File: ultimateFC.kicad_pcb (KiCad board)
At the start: 6 copper layers, 36 x 36 mm, 240 parts, among them J1 USB_B_Micro, SW1 SW_Push, U1 LMR33630CQRNX, U2 TPS62824ADMQ, U3 LMR33620CRNXT, U4 S25FL064L, U5 DPS310, U6 BMI270, U7 STM32H735VGH6, U8 ICM-20602, Y1 CSTNE8M00G550000R0

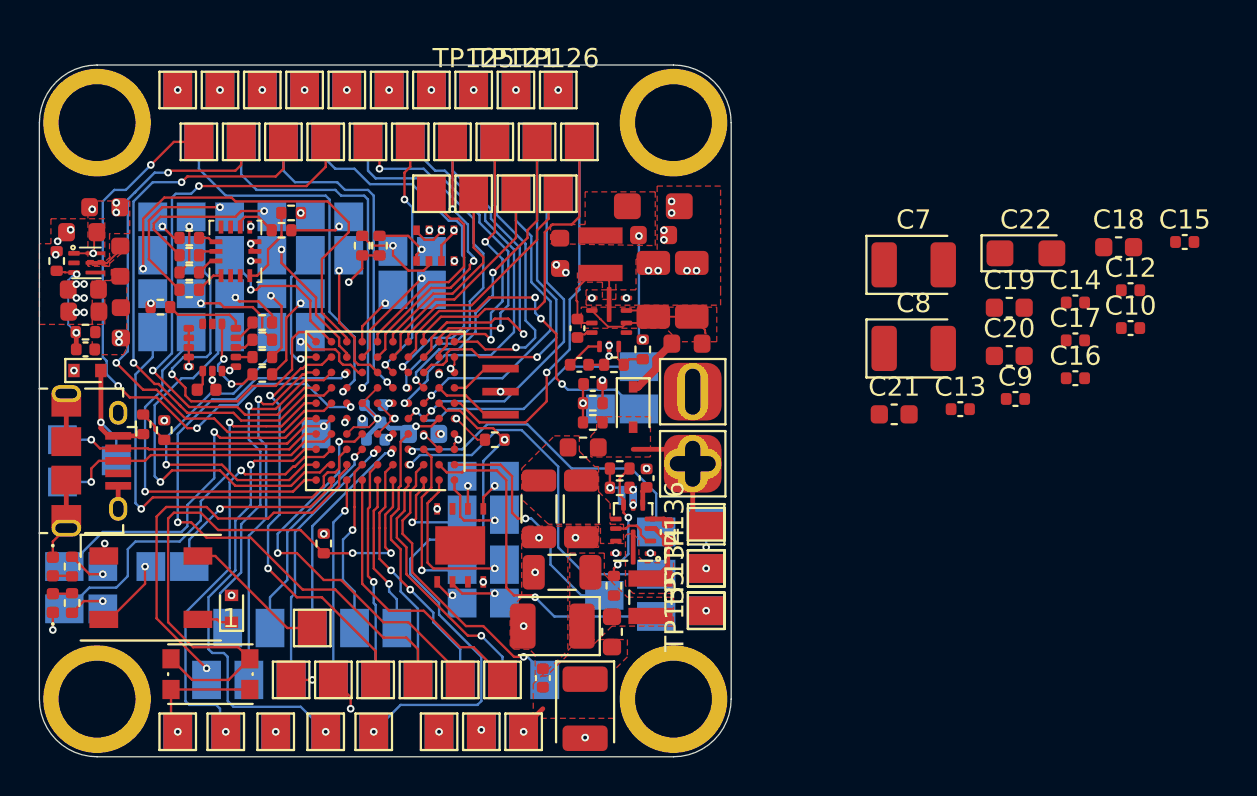
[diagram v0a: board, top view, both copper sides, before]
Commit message: layout tweaks
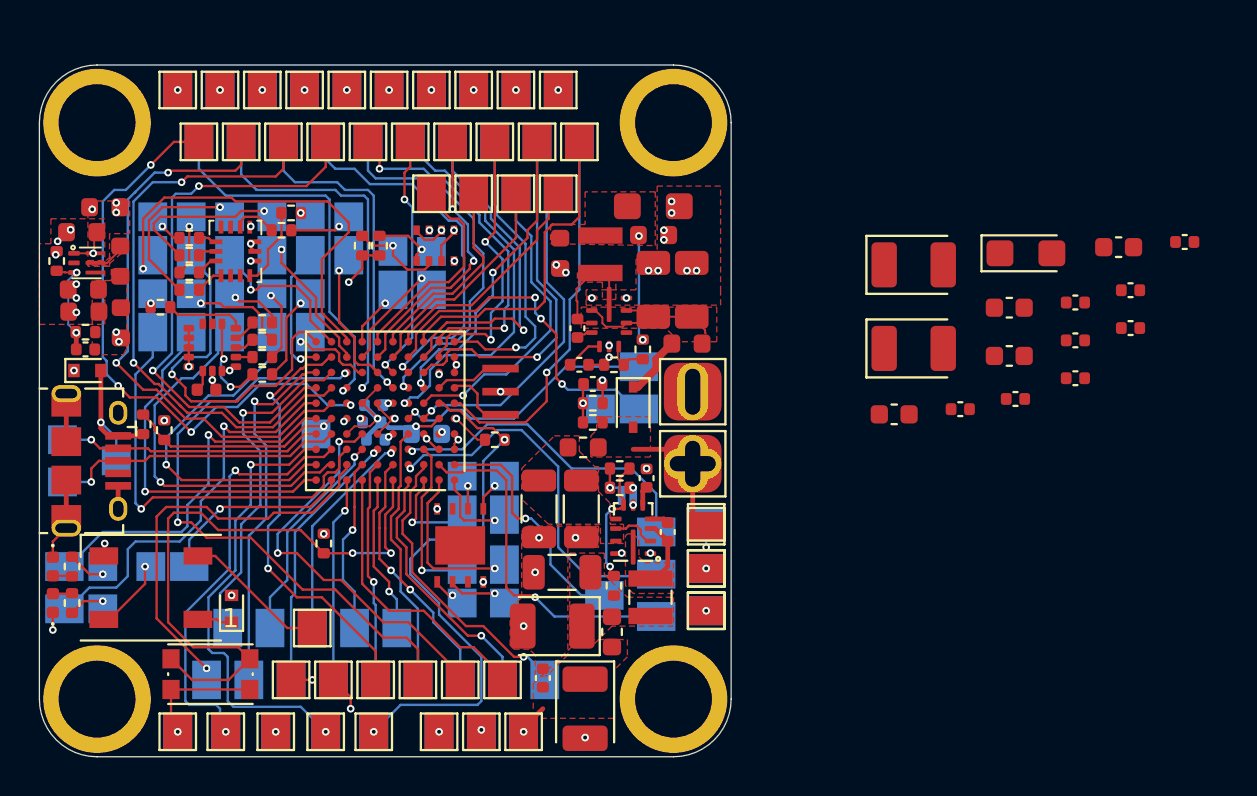
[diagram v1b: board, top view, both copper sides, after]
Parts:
- moved L4 0.15 mm to (117.2, 116.2)
- turned Y1 to 90 degrees
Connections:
- U7 pad A5: Net-(U7-PadA5) -> Net-(R11-Pad1)
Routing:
- net Net-(U7-PadG1): track 2.81 -> 3.47 mm
- net GND: track 19.6 -> 19.5 mm, vias 57 -> 54
